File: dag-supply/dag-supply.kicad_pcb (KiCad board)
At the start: 2 copper layers, 55.9 x 43.2 mm, 14 parts, among them J1 9V1, J2 5V, J3 12V, U1 LM7805_TO220

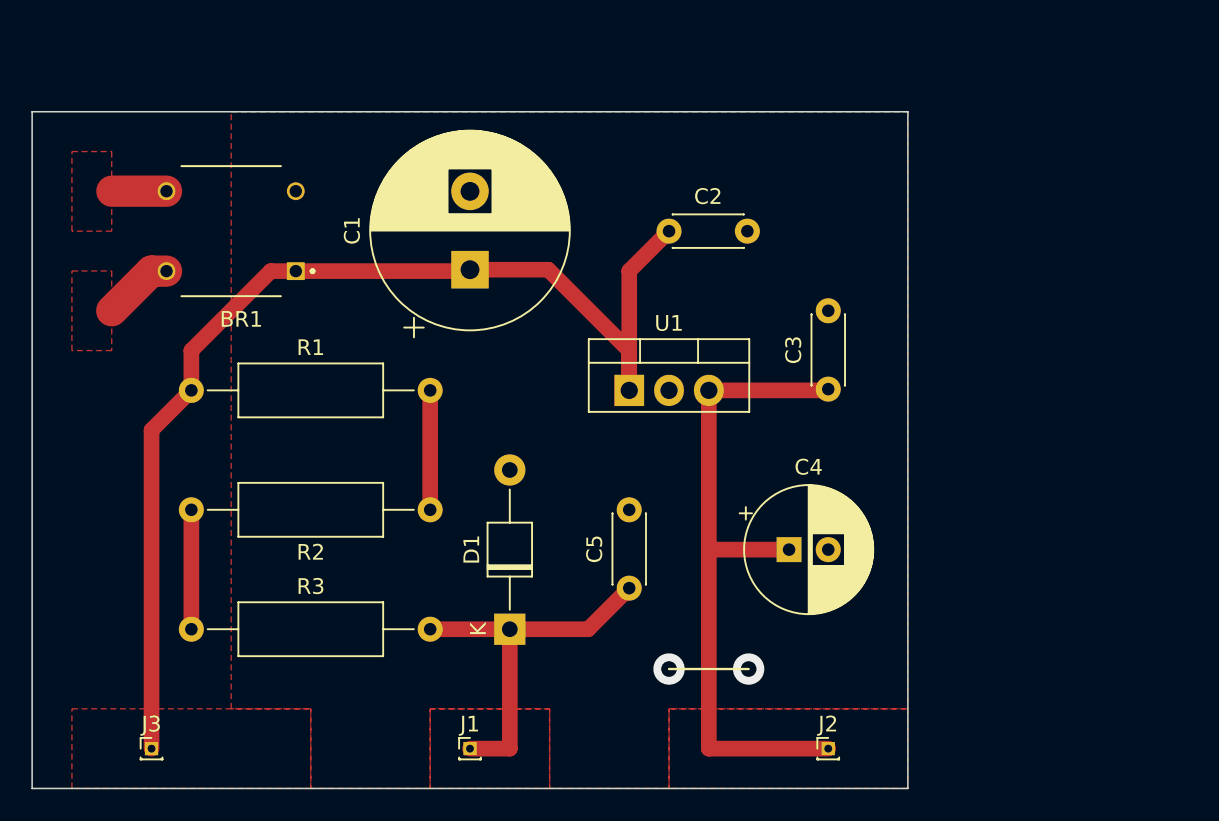
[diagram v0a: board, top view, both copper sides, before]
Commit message: working on pcb
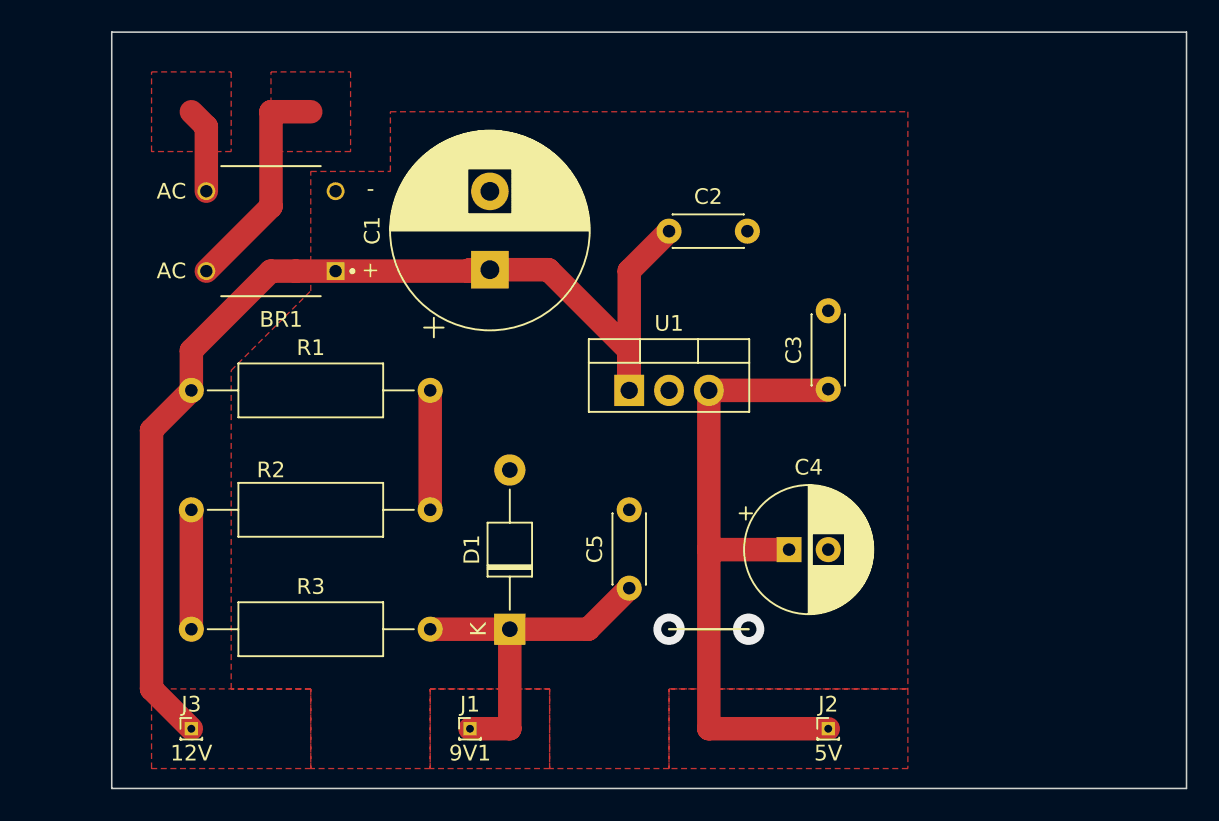
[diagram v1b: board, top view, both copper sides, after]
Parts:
- moved J3 2.84 mm to (55.9, 82.5)
- moved BR1 2.54 mm to (61.0, 50.8)
- moved C1 1.27 mm to (74.9, 53.3)
- moved J1 1.27 mm to (73.7, 82.5)
- moved J2 1.27 mm to (96.5, 82.5)
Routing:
- net VAC: track 8.04 -> 19.9 mm
- net +9V: track 23.9 -> 22.7 mm
- net +5V: track 43.3 -> 42.0 mm
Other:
- board size 55.9 x 43.2 mm -> 68.6 x 48.3 mm
